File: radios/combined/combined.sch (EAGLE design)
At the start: 14 parts

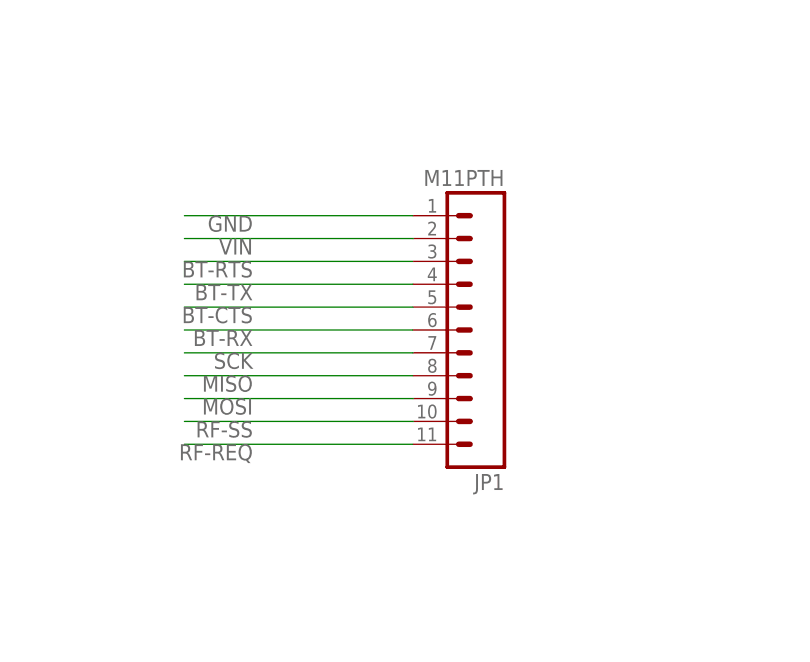
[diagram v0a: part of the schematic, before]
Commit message: about to cut board
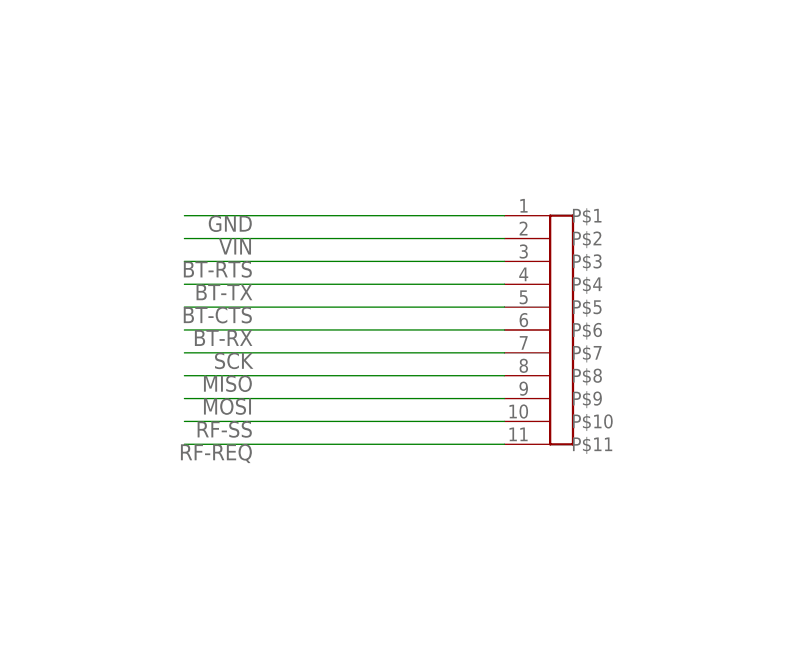
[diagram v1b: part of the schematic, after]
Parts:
- removed JP1: M11PTH, SparkFun-Connectors:M11PTH
- added U$5: HEADER-11, ITP_Lab:HEADER-11
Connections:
- net BT-CTS: now also U$5.P$5; no longer JP1.5
- net BT-RTS: now also U$5.P$3; no longer JP1.3
- net BT-RX: now also U$5.P$6; no longer JP1.6
- net BT-TX: now also U$5.P$4; no longer JP1.4
- net GND: now also U$5.P$1; no longer JP1.1
- net MISO: now also U$5.P$8; no longer JP1.8
- net MOSI: now also U$5.P$9; no longer JP1.9
- net RF-REQ: now also U$5.P$11; no longer JP1.11
- net RF-SS: now also U$5.P$10; no longer JP1.10
- net SCK: now also U$5.P$7; no longer JP1.7
- net VIN: now also U$5.P$2; no longer JP1.2
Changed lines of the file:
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@@
 <part name="CLOCK" library="ITP_Lab" deviceset="PAD" device=""/>
 <part name="VCC" library="ITP_Lab" deviceset="PAD" device=""/>
-<part name="JP1" library="SparkFun-Connectors" deviceset="M11" device="PTH"/>
+<part name="U$5" library="ITP_Lab" deviceset="HEADER-11" device=""/>
 </parts>
 <sheets>
@@
 <instance part="CLOCK" gate="G$1" x="254" y="152.4"/>
 <instance part="VCC" gate="G$1" x="83.82" y="218.44" rot="R90"/>
-<instance part="JP1" gate="G$1" x="121.92" y="142.24" rot="R180"/>
+<instance part="U$5" gate="G$1" x="127" y="142.24"/>
 </instances>
 <busses>
@@
 </segment>
 <segment>
-<wire x1="111.76" y1="154.94" x2="86.36" y2="154.94" width="0.1524" layer="91"/>
+<wire x1="121.92" y1="154.94" x2="86.36" y2="154.94" width="0.1524" layer="91"/>
 <label x="93.98" y="154.94" size="1.778" layer="95" rot="R180"/>
-<pinref part="JP1" gate="G$1" pin="1"/>
+<pinref part="U$5" gate="G$1" pin="P$1"/>
 </segment>
 <segment>
@@
 <net name="VIN" class="0">
 <segment>
-<wire x1="111.76" y1="152.4" x2="86.36" y2="152.4" width="0.1524" layer="91"/>
+<wire x1="121.92" y1="152.4" x2="86.36" y2="152.4" width="0.1524" layer="91"/>
 <label x="93.98" y="152.4" size="1.778" layer="95" rot="R180"/>
-<pinref part="JP1" gate="G$1" pin="2"/>
+<pinref part="U$5" gate="G$1" pin="P$2"/>
 </segment>
 <segment>
@@
 </segment>
 <segment>
-<wire x1="111.76" y1="144.78" x2="86.36" y2="144.78" width="0.1524" layer="91"/>
+<wire x1="121.92" y1="144.78" x2="86.36" y2="144.78" width="0.1524" layer="91"/>
 <label x="93.98" y="144.78" size="1.778" layer="95" rot="R180"/>
-<pinref part="JP1" gate="G$1" pin="5"/>
+<pinref part="U$5" gate="G$1" pin="P$5"/>
 </segment>
 </net>
@@
 </segment>
 <segment>
-<wire x1="111.76" y1="147.32" x2="86.36" y2="147.32" width="0.1524" layer="91"/>
+<wire x1="121.92" y1="147.32" x2="86.36" y2="147.32" width="0.1524" layer="91"/>
 <label x="93.98" y="147.32" size="1.778" layer="95" rot="R180"/>
-<pinref part="JP1" gate="G$1" pin="4"/>
+<pinref part="U$5" gate="G$1" pin="P$4"/>
 </segment>
 </net>
@@
 </segment>
 <segment>
-<wire x1="111.76" y1="142.24" x2="86.36" y2="142.24" width="0.1524" layer="91"/>
+<wire x1="121.92" y1="142.24" x2="86.36" y2="142.24" width="0.1524" layer="91"/>
 <label x="93.98" y="142.24" size="1.778" layer="95" rot="R180"/>
-<pinref part="JP1" gate="G$1" pin="6"/>
+<pinref part="U$5" gate="G$1" pin="P$6"/>
 </segment>
 </net>
@@
 </segment>
 <segment>
-<wire x1="111.76" y1="149.86" x2="86.36" y2="149.86" width="0.1524" layer="91"/>
+<wire x1="121.92" y1="149.86" x2="86.36" y2="149.86" width="0.1524" layer="91"/>
 <label x="93.98" y="149.86" size="1.778" layer="95" rot="R180"/>
-<pinref part="JP1" gate="G$1" pin="3"/>
+<pinref part="U$5" gate="G$1" pin="P$3"/>
 </segment>
 </net>
@@
 </segment>
 <segment>
-<wire x1="111.76" y1="129.54" x2="86.36" y2="129.54" width="0.1524" layer="91"/>
+<wire x1="121.92" y1="129.54" x2="86.36" y2="129.54" width="0.1524" layer="91"/>
 <label x="93.98" y="129.54" size="1.778" layer="95" rot="R180"/>
-<pinref part="JP1" gate="G$1" pin="11"/>
+<pinref part="U$5" gate="G$1" pin="P$11"/>
 </segment>
 </net>
@@
 </segment>
 <segment>
-<wire x1="111.76" y1="132.08" x2="86.36" y2="132.08" width="0.1524" layer="91"/>
+<wire x1="121.92" y1="132.08" x2="86.36" y2="132.08" width="0.1524" layer="91"/>
 <label x="93.98" y="132.08" size="1.778" layer="95" rot="R180"/>
-<pinref part="JP1" gate="G$1" pin="10"/>
+<pinref part="U$5" gate="G$1" pin="P$10"/>
 </segment>
 </net>
@@
 </segment>
 <segment>
-<wire x1="111.76" y1="134.62" x2="86.36" y2="134.62" width="0.1524" layer="91"/>
+<wire x1="121.92" y1="134.62" x2="86.36" y2="134.62" width="0.1524" layer="91"/>
 <label x="93.98" y="134.62" size="1.778" layer="95" rot="R180"/>
-<pinref part="JP1" gate="G$1" pin="9"/>
+<pinref part="U$5" gate="G$1" pin="P$9"/>
 </segment>
 </net>
@@
 </segment>
 <segment>
-<wire x1="111.76" y1="137.16" x2="86.36" y2="137.16" width="0.1524" layer="91"/>
+<wire x1="121.92" y1="137.16" x2="86.36" y2="137.16" width="0.1524" layer="91"/>
 <label x="93.98" y="137.16" size="1.778" layer="95" rot="R180"/>
-<pinref part="JP1" gate="G$1" pin="8"/>
+<pinref part="U$5" gate="G$1" pin="P$8"/>
 </segment>
 </net>
@@
 </segment>
 <segment>
-<wire x1="111.76" y1="139.7" x2="86.36" y2="139.7" width="0.1524" layer="91"/>
+<wire x1="121.92" y1="139.7" x2="86.36" y2="139.7" width="0.1524" layer="91"/>
 <label x="93.98" y="139.7" size="1.778" layer="95" rot="R180"/>
-<pinref part="JP1" gate="G$1" pin="7"/>
-</segment>
-</net>
+<pinref part="U$5" gate="G$1" pin="P$7"/>
+</segment>
+</net>
